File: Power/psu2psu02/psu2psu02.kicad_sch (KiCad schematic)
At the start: 46 parts, among them Q1 740, Q2 740, T1 BC817, T2 BC807, U1 TL494IDR, U2 IR2113S, U3 PC817

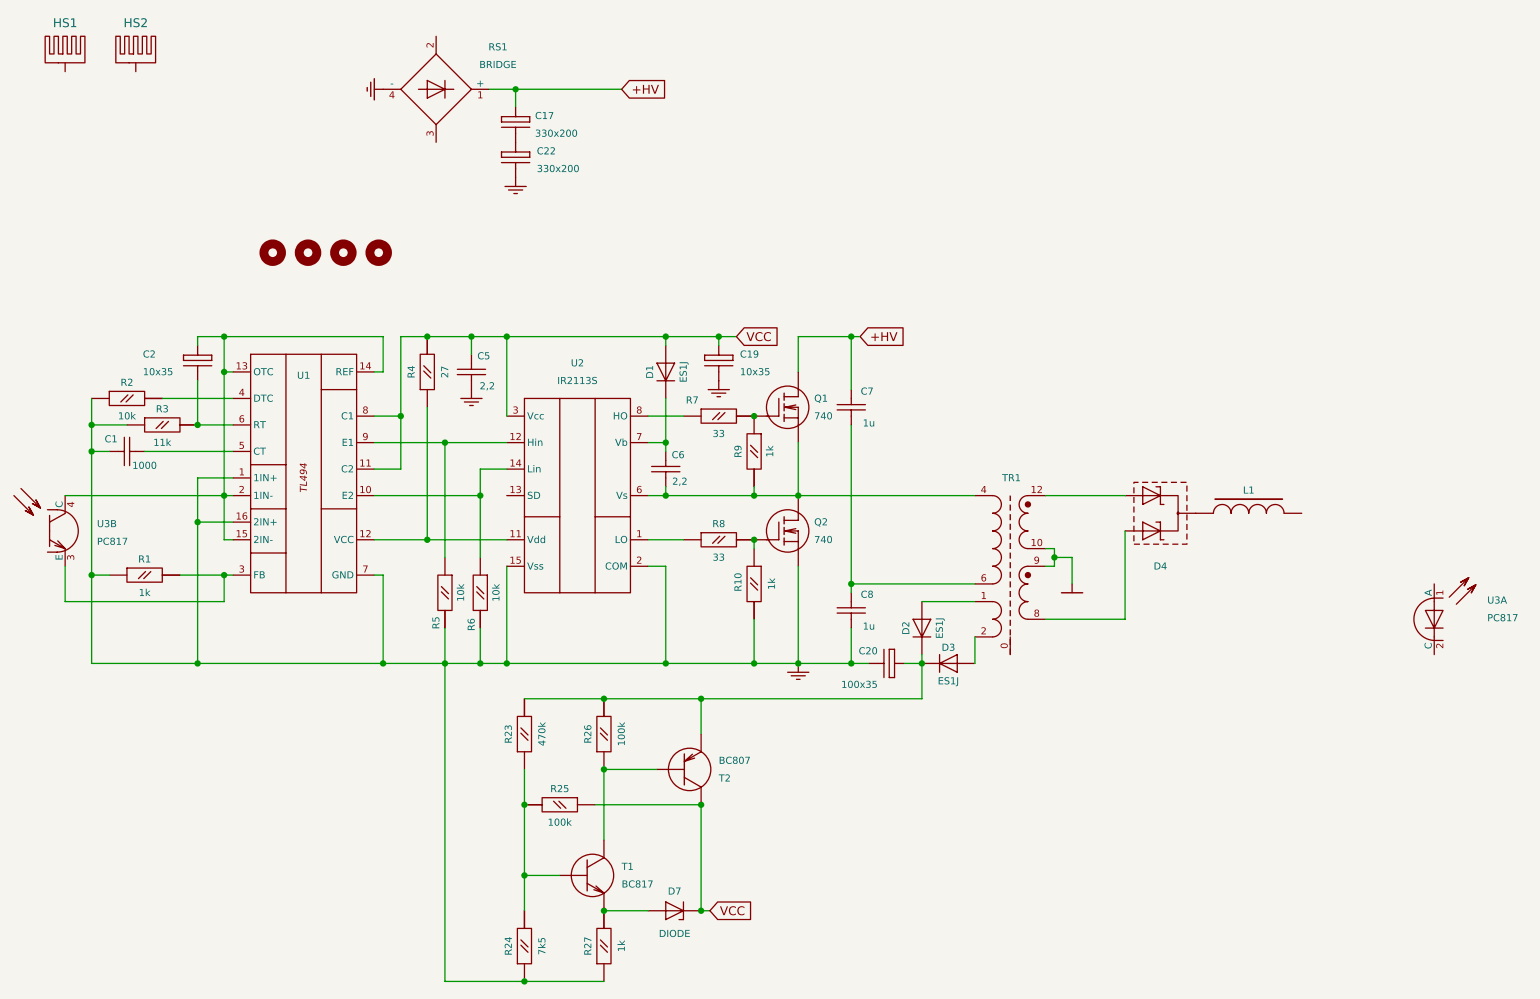
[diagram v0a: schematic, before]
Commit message: op
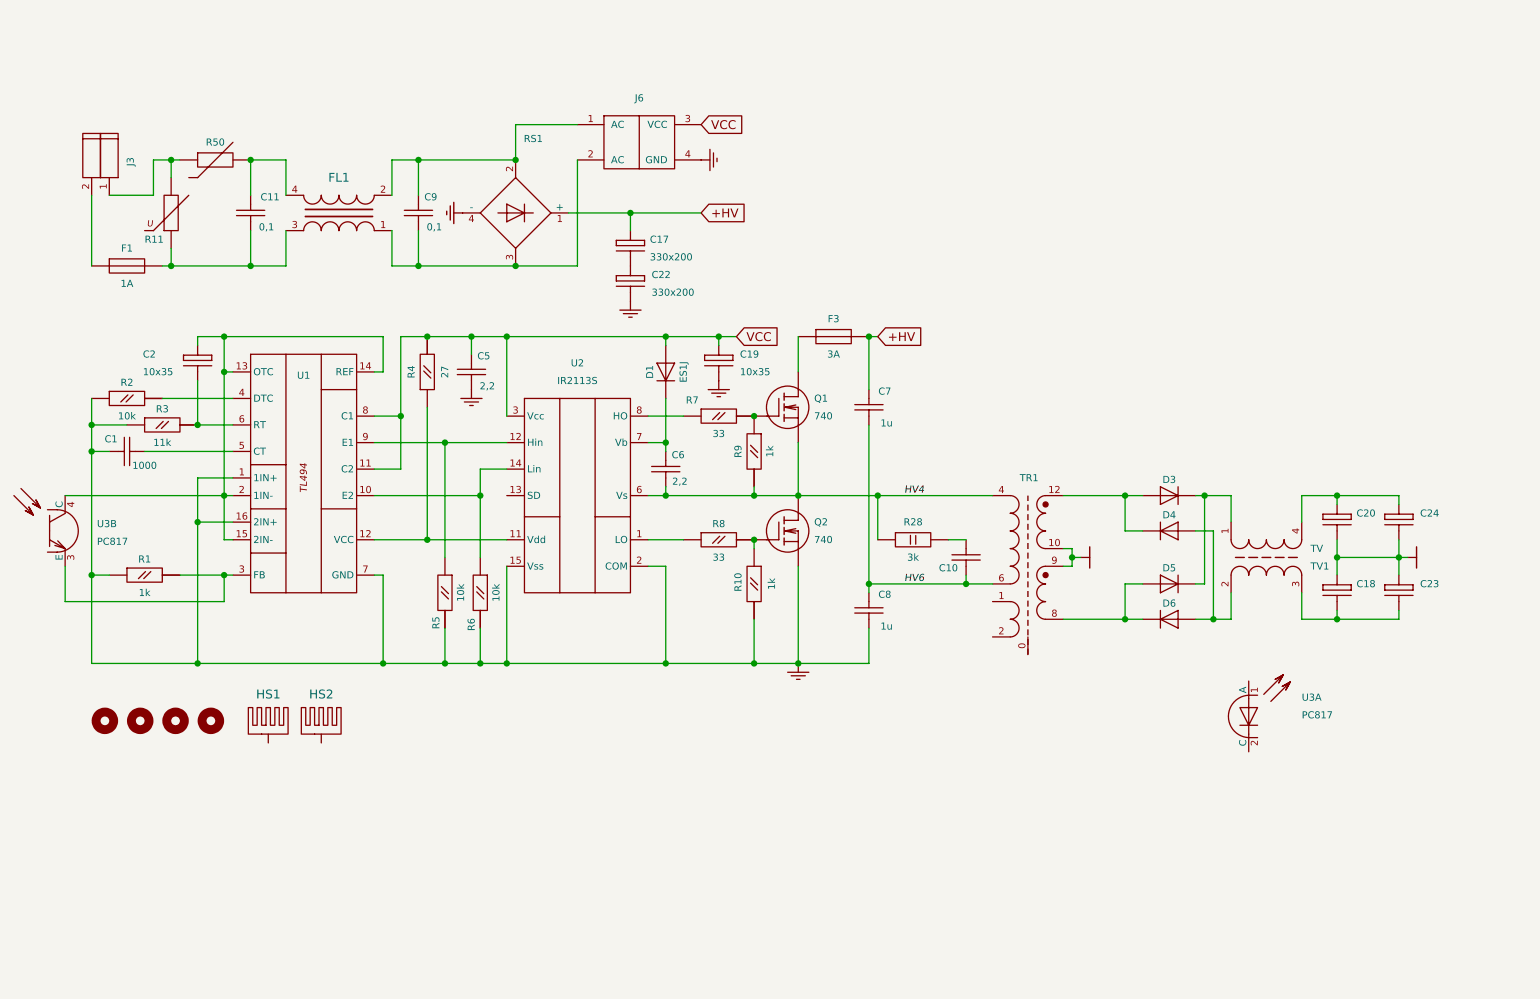
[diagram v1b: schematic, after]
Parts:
- removed D2, D3: ES1J, Diode_SMD:D_SMA, symbol _aa40_diodes:DIODE
- removed D4: ~, Package_TO_SOT_THT:TO-220-3_Vertical, symbol _aa40_diodes:MBR20100CT
- removed D7: DIODE, Diode_SMD:D_MiniMELF, symbol _aa40_diodes:ZENER
- removed L1: LFERR, _aTransformers:DRO05-FLEX-200A, symbol _aa40_inductors:LFERR
- removed R23: 470k, Resistor_SMD:R_1206_3216Metric, symbol _aa40_resistors:R_RES_0.125W
- removed R24: 7k5, Resistor_SMD:R_1206_3216Metric, symbol _aa40_resistors:R_RES_0.125W
- removed R25, R26: 100k, Resistor_SMD:R_1206_3216Metric, symbol _aa40_resistors:R_RES_0.125W
- removed R27: 1k, Resistor_SMD:R_1206_3216Metric, symbol _aa40_resistors:R_RES_0.125W
- removed T1: BC817, Package_TO_SOT_SMD:SOT-23, symbol _aa40_transistors:BC817-40
- removed T2: BC807, Package_TO_SOT_SMD:SOT-23, symbol _aa40_transistors:BC807-40
- added C10: 4n7, Capacitor_THT:C_Disc_D4.3mm_W1.9mm_P5.00mm, symbol _aa40_capacitors:C_CAP
- added C11, C9: 0,1, _aCapa:C_Rect_06-L16P15W5.8, symbol _aa40_capacitors:C_CAP
- added C18, C23, C24: 1, Capacitor_THT:CP_Radial_D16.0mm_P7.50mm, symbol _aa40_capacitors:C_CAP_PLUS1
- added D3, D4, D5, D6: SF10A400H, Package_TO_SOT_THT:TO-220-2_Vertical, symbol _aa40_diodes:SF10A400H
- added F1: 1A, Fuse:Fuseholder_Clip-5x20mm_Littelfuse_100_Inline_P20.50x4.60mm_D1.30mm_Horizontal, symbol _aa40_misc:FUSE
- added F3: 3A, Fuse:Fuse_Littelfuse_395Series, symbol _aa40_misc:FUSE
- added FL1: FEMI-FLEX01, _aTransformers:EMIF02-FLEX, symbol _aa40_transformers:FEMI-FLEX01
- added J3: Conn_2pin01, Connector_Phoenix_GMSTB:PhoenixContact_GMSTBVA_2,5_2-G-7,62_1x02_P7.62mm_Vertical, symbol _aa40_connectors:Conn_2pin01
- added J6: ACDC_China-01, _aModules:ACDC_China-04, symbol _aa40_misc:ACDC_China-01
- added R11: 07K180, Varistor:RV_Disc_D12mm_W3.9mm_P7.5mm, symbol _aa40_resistors:R_VAR1
- added R28: 3k, _aResistors:RES2WV01, symbol _aa40_resistors:R_RES_2.0W
- added R50: t°, Varistor:RV_Disc_D12mm_W3.9mm_P7.5mm, symbol _aa40_resistors:R_TERM1
- added TV1: TV, _aTransformers:DRO05-FLEX-200A, symbol _aa40_transformers:TV2
- C17, C22: footprint Capacitor_THT:CP_Radial_D18.0mm_P7.50mm -> Capacitor_THT:CP_Radial_D22.0mm_P10.00mm_SnapIn
- C20: value 100x35 -> 1; footprint Capacitor_THT:CP_Radial_D6.3mm_P2.50mm -> Capacitor_THT:CP_Radial_D16.0mm_P7.50mm
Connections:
- net +HV: now also F3.2; no longer Q1.2 (D)
- net GND: now also C20.2, C18.1, C23.1, C24.2
- net GND2: now also J6.4 (GND); no longer C20.2
- net VCC: now also J6.3 (VCC)
- net HV6: now reaches C7.1, C8.2, TR1.6
- net HV6: now also C10.1
- net at C20.1: now also C24.1, TV1.4
- net HV4: now reaches C6.1, Q1.3 (S), Q2.2 (D), R9.2, TR1.4, U2.6 (Vs)
- net HV4: now also R28.1
- net at TR1.7, TR1.8: now also D5.2 (A), D6.1 (C)
- net at TR1.11, TR1.12: now also D3.2 (A), D4.1 (C)
- net at RS1.2: now also C9.2, FL1.2, J6.1 (AC)
- net at RS1.3: now also C9.1, FL1.1, J6.2 (AC)
- new net: D4.2 (A), D6.2 (A), TV1.2
- new net: C11.1, F1.2, FL1.3, R11.1
- new net: J3.1, R11.2, R50.1
- new net: D3.1 (C), D5.1 (C), TV1.1
- new net: F1.1, J3.2
- new net: C11.2, FL1.4, R50.2
- new net: C10.2, R28.2
- new net: C18.2, C23.2, TV1.3
- new net: F3.1, Q1.2 (D)
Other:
- moved on the sheet: C17, C22, C7, C8, HS1, HS2, RS1, TR1, U3A
